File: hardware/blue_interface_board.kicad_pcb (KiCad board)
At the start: 4 copper layers, 70 x 70 mm, 130 parts, among them J1 arm connector, J10 I2C, J2 USB_B_Micro, J3 ESTOP, J4 PWR, J5 Conn_ARM_JTAG_SWD_10, J6 logic-side RS485 debug/expans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, J7 FAN, J8 power-side RS485 debug/expans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, J9 DEBUG, Q1 MMBT5401LT1G, Q2 PSMN4R8-100BSEJ, Q3 MMBT3904, Q5 PSMN4R8-100BSEJ, Q7 NTS4001NT1G, U1 93LCxxB, U10 LMZ21700SIL, U11 LMZ21700SIL, U2 FT232H, U3 ADM2682E, U4 TPD2E2U06DCK, U5 TPD2E2U06DCK, U6 LM5066, U7 STM32L071KZT6, U8 LM46000, U9 FAN3111E, Y1 12MHz

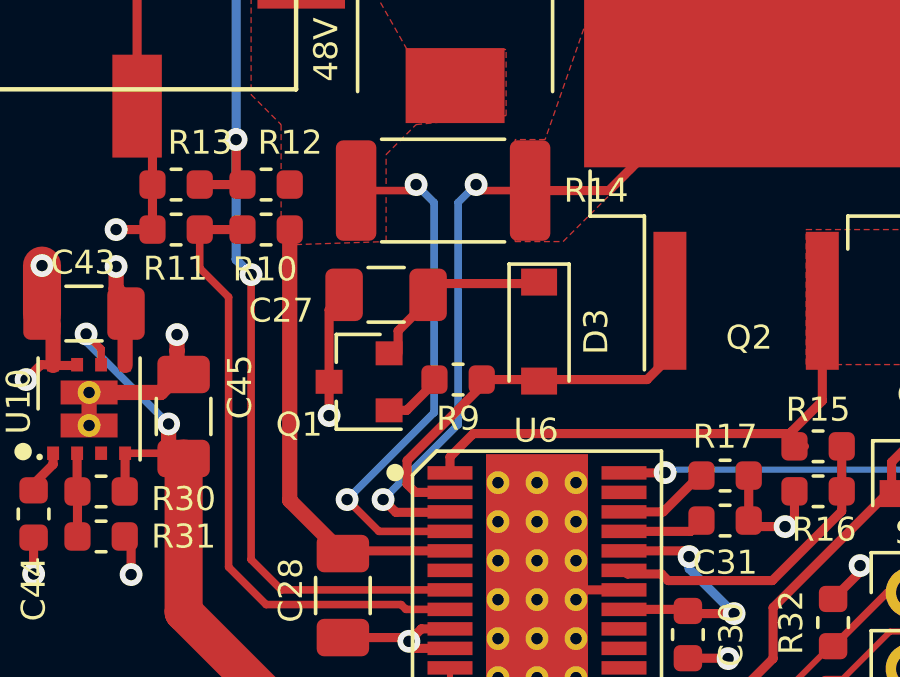
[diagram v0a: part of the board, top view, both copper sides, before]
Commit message: Adding ERD resistors to layout.
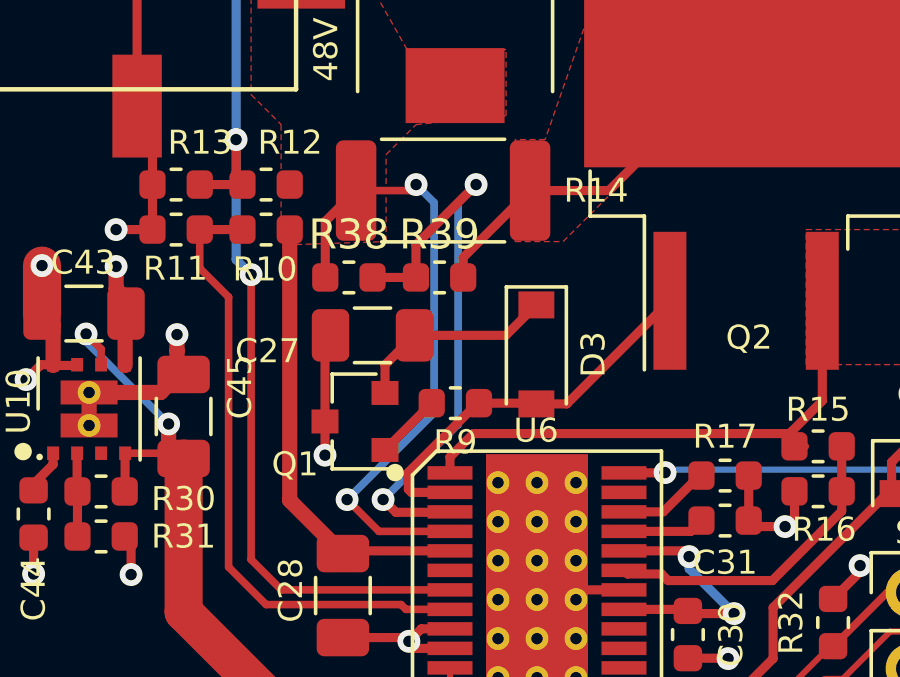
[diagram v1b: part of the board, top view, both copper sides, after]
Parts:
- added R38: 10, Resistor_SMD:R_0603_1608Metric, F.Cu at (100.8, 108.1)
- added R39: 2, Resistor_SMD:R_0603_1608Metric, F.Cu at (103.8, 108.1)
- C31: value 100n -> 1u
- R14: value 15m -> 5m
- R15: value 140k -> 240k
- R16: value 21k -> 13.3k
- R17: value 21k -> 300k
- moved C27 1.42 mm to (101.5, 110.0)
- moved Q1 1.33 mm to (101.0, 112.9)
- moved R9 0.79 mm to (104.3, 112.3)
- moved D3 0.77 mm to (107.0, 110.7)
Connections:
- U6 pad 3: Net-(Q2-Pad2) -> Net-(R38-Pad2)
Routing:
- net Net-(R38-Pad2): track 0.00 -> 19.6 mm, vias 0 -> 2
- net Net-(Q2-Pad2): track 24.3 -> 12.1 mm, vias 2 -> 0
- net /Power/VIN: track 33.0 -> 36.4 mm
- net /Power/GATE: track 14.5 -> 13.1 mm
- net Net-(C27-Pad1): track 5.79 -> 6.81 mm
- net GND: track 110.0 -> 109.3 mm

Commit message: Removing external resistor divider.
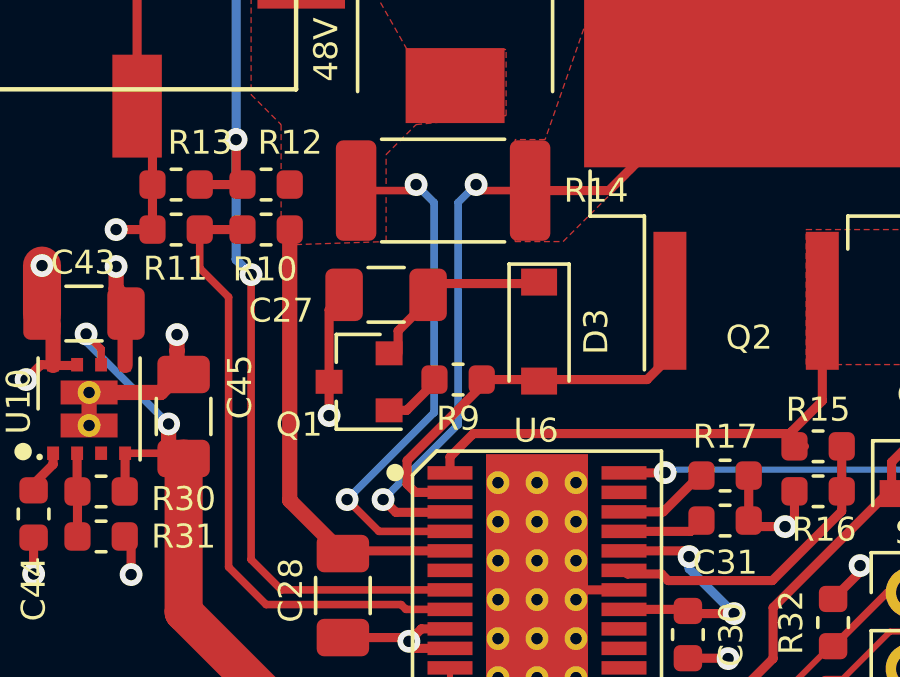
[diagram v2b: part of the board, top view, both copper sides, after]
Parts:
- removed R38: 10, Resistor_SMD:R_0603_1608Metric
- removed R39: 2, Resistor_SMD:R_0603_1608Metric
- C31: value 1u -> 100n
- R14: value 5m -> 15m
- R15: value 240k -> 140k
- R16: value 13.3k -> 21k
- R17: value 300k -> 21k
- moved C27 1.42 mm to (102.0, 108.7)
- moved Q1 1.33 mm to (101.1, 111.6)
- moved R9 0.79 mm to (104.4, 111.5)
- moved D3 0.77 mm to (107.1, 109.9)
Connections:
- U6 pad 3: Net-(R38-Pad2) -> Net-(Q2-Pad2)
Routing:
- net Net-(R38-Pad2): track 19.6 -> 0.00 mm, vias 2 -> 0
- net Net-(Q2-Pad2): track 12.1 -> 24.3 mm, vias 0 -> 2
- net /Power/VIN: track 36.4 -> 33.0 mm
- net /Power/GATE: track 13.1 -> 14.5 mm
- net Net-(C27-Pad1): track 6.81 -> 5.79 mm
- net GND: track 109.3 -> 110.0 mm
